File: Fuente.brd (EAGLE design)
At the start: 100 x 100.2 mm, 39 parts, among them U3 LCD-16X28X2

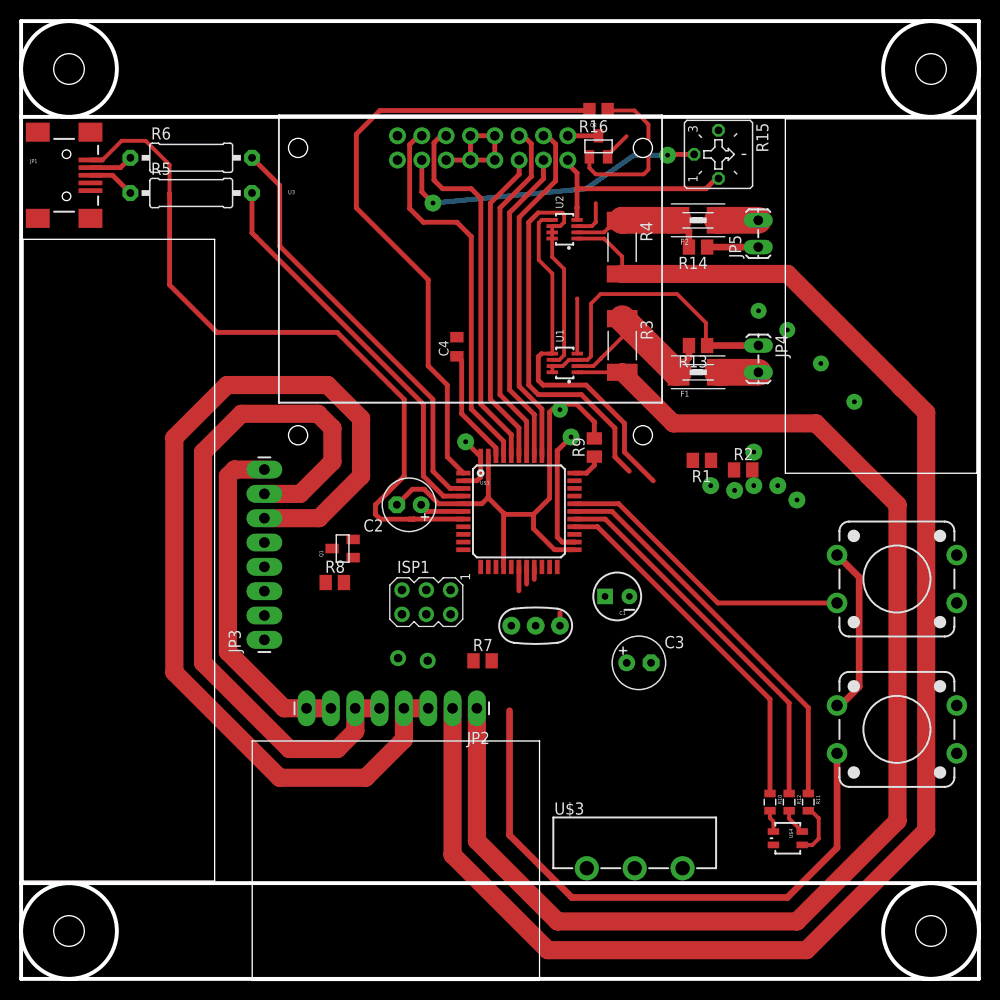
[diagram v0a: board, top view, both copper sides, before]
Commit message: updated pcb and sch
ready for first print
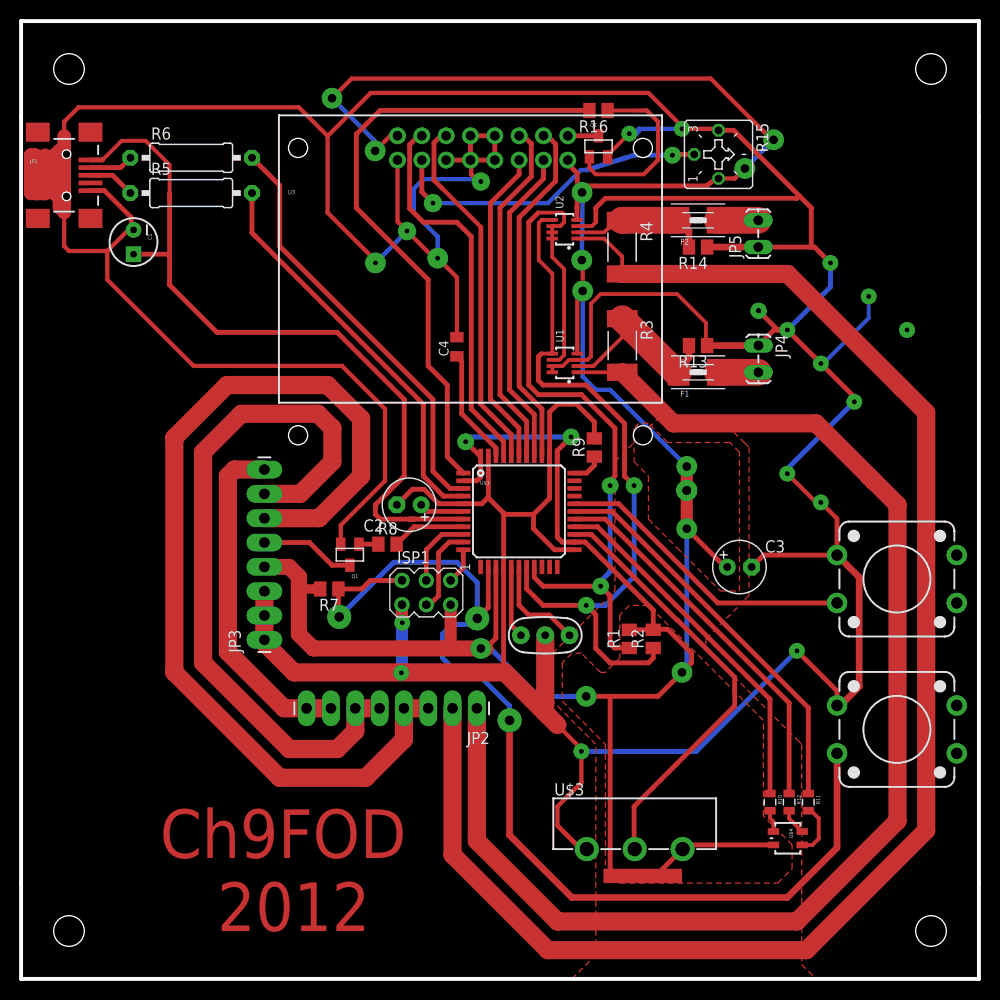
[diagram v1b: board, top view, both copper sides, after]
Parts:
- moved C1 62.6 mm to (11.7, 66.9), turned to 270 degrees
- moved R1 20.1 mm to (63.5, 25.5), turned to 90 degrees
- moved R2 20.0 mm to (66.0, 25.5), turned to 90 degrees
- moved R7 17.7 mm to (32.2, 30.7), turned to 180 degrees
- moved C3 14.5 mm to (75.0, 33.0)
- moved R8 6.80 mm to (38.3, 35.4)
- moved U$3 2.00 mm to (64.1, 3.55)
- moved Y1 1.41 mm to (54.7, 25.9)
- moved ISP1 1.00 mm to (42.3, 30.3)
- moved Q1 0.99 mm to (34.3, 34.3), turned to 180 degrees
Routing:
- net GND: track 127.1 -> 577.2 mm, vias 5 -> 20
- net 5V: track 47.0 -> 315.1 mm, vias 3 -> 16
- net R1: track 61.9 -> 115.5 mm, vias 0 -> 3
- net CTRL: track 0.00 -> 45.3 mm
- net SCL: track 39.7 -> 75.9 mm, vias 0 -> 2
- net SDA: track 56.1 -> 83.8 mm, vias 0 -> 2
- net N$24: track 0.00 -> 13.5 mm, vias 1 -> 0
- net EN: track 0.00 -> 9.91 mm
- net N$20: track 0.00 -> 9.57 mm, vias 1 -> 0
- net MOSI: track 0.00 -> 9.22 mm
- net SCK: track 0.00 -> 7.74 mm
- net ON: track 0.00 -> 7.73 mm
- net N$13: track 0.01 -> 7.55 mm
- net N$12: track 3.85 -> 10.6 mm
- net N$23: track 0.00 -> 6.41 mm, vias 1 -> 0
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- added copper zone on layer 1, net 5V
- added copper zone on layer 1, net GND
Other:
- board size 100 x 100.2 mm -> 100 x 100 mm
- board text added: "Ch9FOD 2012"
